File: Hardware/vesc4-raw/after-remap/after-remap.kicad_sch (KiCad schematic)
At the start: 26 parts, among them K1 SERVO, P1 HALL/Encoder, P101 CANBUS, P3 PWR_COMM, P4 IN+, P5 IN-, P6 MOTOR1, P7 MOTOR2, P9 MOTOR3

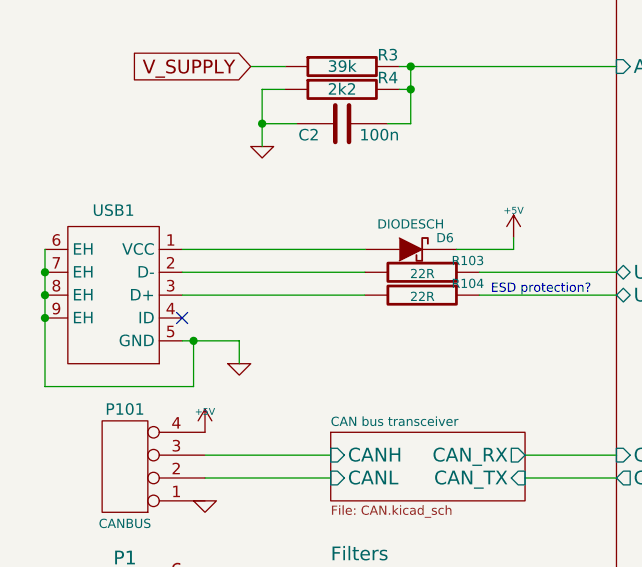
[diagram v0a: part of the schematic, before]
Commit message: checkpoint sebelum ngetrace usb
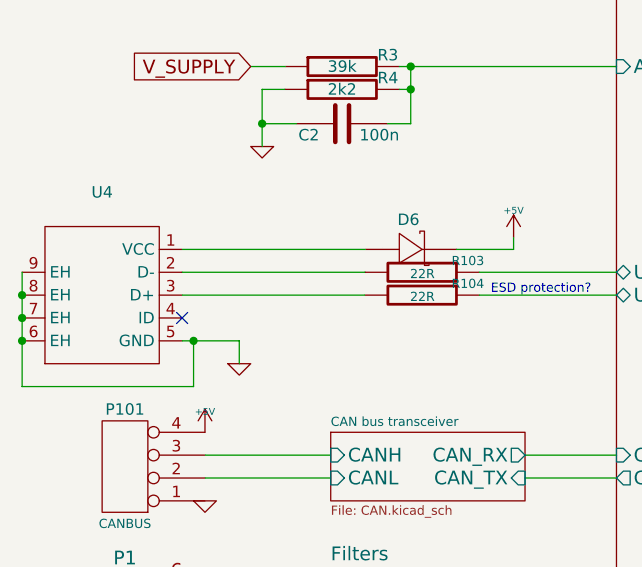
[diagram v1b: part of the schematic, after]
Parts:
- removed D6: DIODESCH, Diodes_SMD:SMA_Handsoldering, symbol vesc4-legacy:DIODESCH_2
- removed USB1: ~, EasyEDA_Lib:MICRO-USB-SMD_HX-USB-MICRO-XNJ-JB, symbol EasyEDA_Lib:HX USB-MICR XNJ ZB
- added D6: ~, EasyEDA_Lib:SMA_L4.2-W2.6-LS5.1-RD, symbol EasyEDA_Lib:SS110_C379823
- added U4: ~, EasyEDA_Lib:MICRO-USB-SMD_MICROUSB-5P-M, symbol EasyEDA_Lib:MICRO USB 5P贴板公头四脚贴带卡勾
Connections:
- net +5V: now also D6.1 (K)
- net GND: now also U4.5 (GND), U4.6 (EH), U4.7 (EH), U4.8 (EH), U4.9 (EH)
- net at R103.2: now also U4.2 (D-)
- net at R104.2: now also U4.3 (D+)
- new net: D6.2 (A), U4.1 (VCC)
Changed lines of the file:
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@@
 	)
 	(junction
-		(at 160.02 140.97)
+		(at 16.51 82.55)
 		(diameter 0)
 		(color 0 0 0 0)
 	)
 	(junction
-		(at 19.05 80.01)
+		(at 160.02 140.97)
 		(diameter 0)
 		(color 0 0 0 0)
@@
 	)
 	(junction
-		(at 19.05 77.47)
+		(at 16.51 85.09)
 		(diameter 0)
 		(color 0 0 0 0)
@@
 	)
 	(junction
-		(at 19.05 82.55)
+		(at 16.51 80.01)
 		(diameter 0)
 		(color 0 0 0 0)
@@
 	(wire
 		(pts
-			(xy 19.05 77.47) (xy 19.05 80.01)
-		)
-		(stroke
-			(width 0)
-			(type default)
-		)
-	)
-	(wire
-		(pts
 			(xy 199.39 113.03) (xy 195.58 113.03)
 		)
@@
 	(wire
 		(pts
-			(xy 43.18 57.15) (xy 45.72 57.15)
+			(xy 16.51 80.01) (xy 16.51 77.47)
 		)
 		(stroke
@@
 	(wire
 		(pts
-			(xy 19.05 82.55) (xy 19.05 90.17)
+			(xy 43.18 57.15) (xy 45.72 57.15)
 		)
 		(stroke
@@
 	(wire
 		(pts
+			(xy 16.51 82.55) (xy 16.51 80.01)
+		)
+		(stroke
+			(width 0)
+			(type default)
+		)
+	)
+	(wire
+		(pts
 			(xy 72.39 114.3) (xy 82.55 114.3)
 		)
@@
 	(wire
 		(pts
+			(xy 16.51 90.17) (xy 35.56 90.17)
+		)
+		(stroke
+			(width 0)
+			(type default)
+		)
+	)
+	(wire
+		(pts
 			(xy 199.39 107.95) (xy 195.58 107.95)
 		)
@@
 	(wire
 		(pts
-			(xy 19.05 80.01) (xy 19.05 82.55)
+			(xy 147.32 88.9) (xy 157.48 88.9)
 		)
 		(stroke
@@
 	(wire
 		(pts
-			(xy 147.32 88.9) (xy 157.48 88.9)
+			(xy 195.58 77.47) (xy 219.71 77.47)
 		)
 		(stroke
@@
 	(wire
 		(pts
-			(xy 195.58 77.47) (xy 219.71 77.47)
+			(xy 67.31 80.01) (xy 82.55 80.01)
 		)
 		(stroke
@@
 	(wire
 		(pts
-			(xy 67.31 80.01) (xy 82.55 80.01)
+			(xy 16.51 90.17) (xy 16.51 85.09)
 		)
 		(stroke
@@
 		)
 	)
+	(wire
+		(pts
+			(xy 16.51 85.09) (xy 16.51 82.55)
+		)
+		(stroke
+			(width 0)
+			(type default)
+		)
+	)
 	(polyline
 		(pts
@@
 	(wire
 		(pts
-			(xy 19.05 74.93) (xy 19.05 77.47)
-		)
-		(stroke
-			(width 0)
-			(type default)
-		)
-	)
-	(wire
-		(pts
 			(xy 171.45 146.05) (xy 177.8 146.05)
 		)
@@
 	(wire
 		(pts
-			(xy 19.05 90.17) (xy 35.56 90.17)
-		)
-		(stroke
-			(width 0)
-			(type default)
-		)
-	)
-	(wire
-		(pts
 			(xy 207.01 101.6) (xy 219.71 101.6)
 		)
@@
 	)
 	(symbol
-		(lib_id "EasyEDA_Lib:HX USB-MICR XNJ ZB")
-		(at 26.67 80.01 180)
+		(lib_id "EasyEDA_Lib:MICRO USB 5P贴板公头四脚贴带卡勾")
+		(at 26.67 80.01 0)
 		(unit 1)
 		(exclude_from_sim no)
@@
 		(on_board yes)
 		(dnp no)
-		(property "Reference" "USB1"
-			(at 26.67 70.612 0)
+		(fields_autoplaced yes)
+		(property "Reference" "U4"
+			(at 25.4 68.58 0)
 			(effects
 				(font
@@
 		)
 		(property "Value" "~"
-			(at 26.67 71.12 0)
+			(at 25.4 71.12 0)
 			(effects
 				(font
@@
 			)
 		)
-		(property "Footprint" "EasyEDA_Lib:MICRO-USB-SMD_HX-USB-MICRO-XNJ-JB"
+		(property "Footprint" "EasyEDA_Lib:MICRO-USB-SMD_MICROUSB-5P-M"
 			(at 26.67 80.01 0)
 			(effects
@@
 			)
 		)
-		(property "Description" "Connector Type:Micro-B Protocol Standard:USB 2.0 Gender:Female Mounting Type:Surface Mount, Right Angle Number of Contacts:5P Number of Ports:1 Current Rating-Power:1A Voltage Rating:30V Connect-Disconnect Life:3,000 Cycles Supplementary Features:- Center"
-			(at 26.67 80.01 0)
-			(effects
-				(font
-					(size 1.27 1.27)
-				)
-				(hide yes)
-			)
-		)
-		(property "Manufacturer Part" "HX USB-MICR XNJ ZB"
+		(property "Description" ""
 			(at 26.67 80.01 0)
 			(effects
@@
 			)
 		)
-		(property "Manufacturer" "hanxia(韩下)"
+		(property "Manufacturer Part" "micro usb 5p贴板公头四脚贴带卡勾"
 			(at 26.67 80.01 0)
 			(effects
@@
 			)
 		)
-		(property "Supplier Part" "C18357557"
+		(property "Supplier Part" "C9900000761"
 			(at 26.67 80.01 0)
 			(effects
@@
 			)
 		)
-		(property "LCSC Part Name" "Micro-B 母 卧贴"
+		(property "LCSC Part Name" "micro usb 5p贴板公头四脚贴带卡勾"
 			(at 26.67 80.01 0)
 			(effects
@@
 			)
 		)
-		(pin "1"
-		)
-		(pin "6"
+		(pin "9"
 		)
-		(pin "5"
+		(pin "2"
 		)
 		(pin "4"
 		)
-		(pin "3"
+		(pin "8"
 		)
-		(pin "2"
+		(pin "1"
 		)
-		(pin "9"
+		(pin "7"
 		)
-		(pin "8"
+		(pin "6"
 		)
-		(pin "7"
+		(pin "3"
+		)
+		(pin "5"
 		)
 		(instances
 			(project ""
 				(path "/97cdaedc-7981-4798-95b0-56b9c66aae09"
-					(reference "USB1")
+					(reference "U4")
 					(unit 1)
 				)
@@
 	)
 	(symbol
-		(lib_name "DIODESCH_2")
-		(lib_id "vesc4-legacy:DIODESCH_2")
-		(at 59.69 74.93 0)
+		(lib_id "EasyEDA_Lib:SS110_C379823")
+		(at 59.69 74.93 180)
 		(unit 1)
 		(exclude_from_sim no)
@@
 		(dnp no)
 		(property "Reference" "D6"
-			(at 63.5 73.66 0)
+			(at 59.436 71.628 0)
 			(effects
 				(font
-					(size 1.016 1.016)
+					(size 1.27 1.27)
 				)
 			)
 		)
-		(property "Value" "DIODESCH"
-			(at 59.69 72.136 0)
+		(property "Value" "~"
+			(at 60.071 71.12 0)
 			(effects
 				(font
-					(size 1.016 1.016)
+					(size 1.27 1.27)
 				)
 			)
 		)
-		(property "Footprint" "Diodes_SMD:SMA_Handsoldering"
+		(property "Footprint" "EasyEDA_Lib:SMA_L4.2-W2.6-LS5.1-RD"
 			(at 59.69 74.93 0)
 			(effects
 				(font
-					(size 1.524 1.524)
+					(size 1.27 1.27)
 				)
 				(hide yes)
 			)
 		)
-		(property "Datasheet" ""
+		(property "Datasheet" "https://atta.szlcsc.com/upload/public/pdf/source/20190416/C379823_9D66F8781E151C8A4940396CFA0EFE63.pdf"
 			(at 59.69 74.93 0)
 			(effects
 				(font
-					(size 1.524 1.524)
+					(size 1.27 1.27)
 				)
 				(hide yes)
 			)
 		)
-		(property "Description" ""
+		(property "Description" "Forward Voltage (Vf@If):850mV@1A Reverse Voltage (Vr):100V Average Rectified Current (Io):1A"
 			(at 59.69 74.93 0)
 			(effects
@@
 					(size 1.27 1.27)
 				)
+				(hide yes)
+			)
+		)
+		(property "Manufacturer Part" "SS110"
+			(at 59.69 74.93 0)
+			(effects
+				(font
+					(size 1.27 1.27)
+				)
+				(hide yes)
+			)
+		)
+		(property "Supplier Part" "C379823"
+			(at 59.69 74.93 0)
+			(effects
+				(font
+					(size 1.27 1.27)
+				)
+				(hide yes)
+			)
+		)
+		(property "Supplier" "LCSC"
+			(at 59.69 74.93 0)
+			(effects
+				(font
+					(size 1.27 1.27)
+				)
+				(hide yes)
+			)
+		)
+		(property "LCSC Part Name" "电压:100V 电流:1A"
+			(at 59.69 74.93 0)
+			(effects
+				(font
+					(size 1.27 1.27)
+				)
+				(hide yes)
 			)
 		)
@@
 		)
 		(instances
-			(project "after-remap"
+			(project ""
 				(path "/97cdaedc-7981-4798-95b0-56b9c66aae09"
 					(reference "D6")
